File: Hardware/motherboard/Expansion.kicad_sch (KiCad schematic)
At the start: 7 parts, among them J1 345-050-520-202, J10 345-050-520-202, J4 345-050-520-202, J5 345-050-520-202, J6 345-050-520-202, J8 345-050-520-202, J9 345-050-520-202

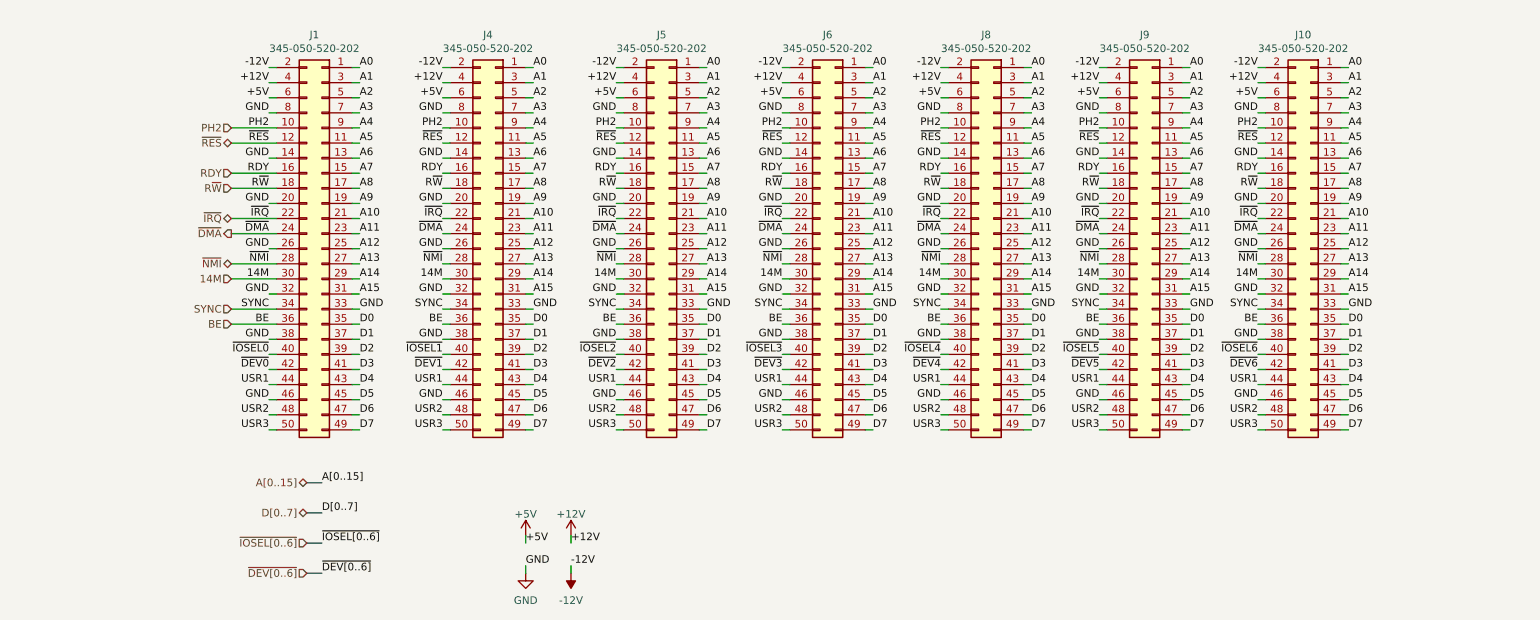
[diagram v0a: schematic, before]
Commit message: Misc hardware work
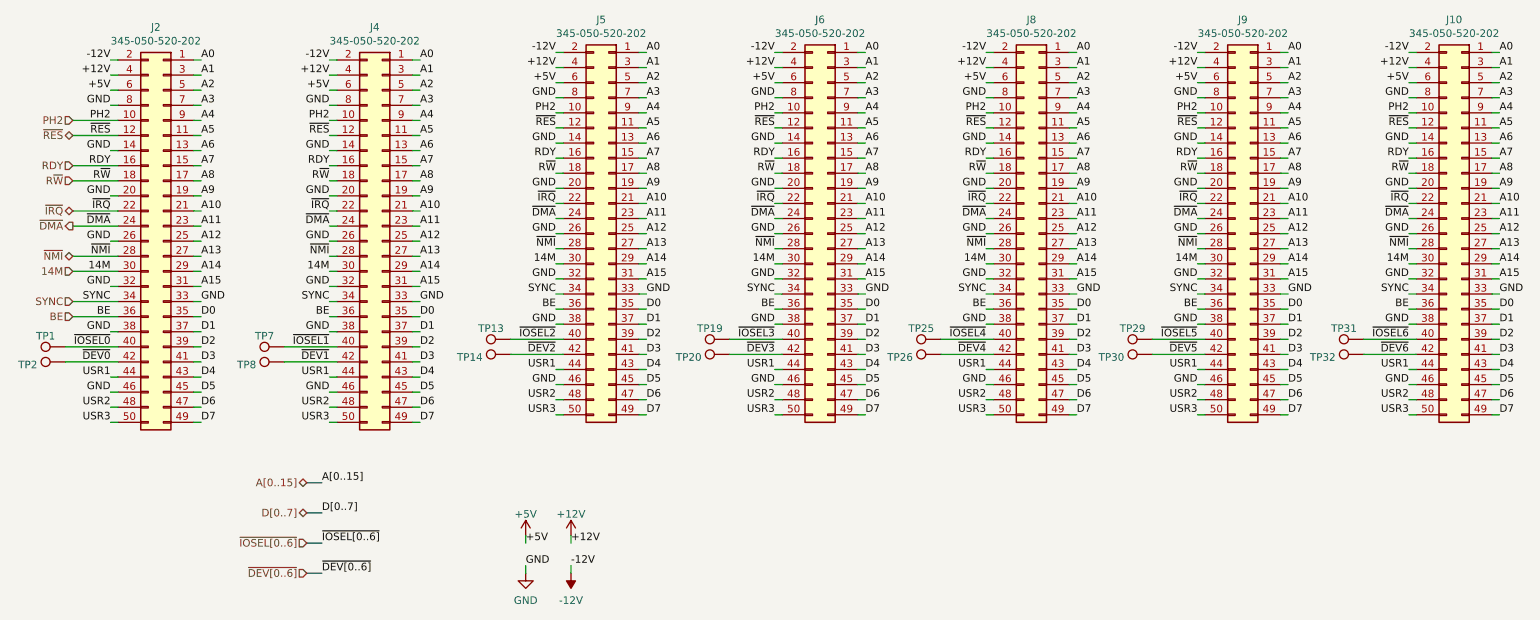
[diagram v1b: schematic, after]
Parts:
- added TP1, TP13, TP14, TP19, TP2, TP20, TP25, TP26, TP29, TP30, TP31, TP32, TP7, TP8: TestPoint, TestPoint:TestPoint_THTPad_D1.5mm_Drill0.7mm, symbol Connector:TestPoint
- renumbered J1 to J2
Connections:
- net ~{DEV0}: now also TP2.1
- net ~{DEV1}: now also TP8.1
- net ~{DEV2}: now also TP14.1
- net ~{DEV3}: now also TP20.1
- net ~{DEV4}: now also TP26.1
- net ~{DEV5}: now also TP30.1
- net ~{DEV6}: now also TP32.1
- net ~{IOSEL0}: now also TP1.1
- net ~{IOSEL1}: now also TP7.1
- net ~{IOSEL2}: now also TP13.1
- net ~{IOSEL3}: now also TP19.1
- net ~{IOSEL4}: now also TP25.1
- net ~{IOSEL5}: now also TP29.1
- net ~{IOSEL6}: now also TP31.1
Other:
- moved on the sheet: J10, J2, J4, J5, J6, J8, J9
